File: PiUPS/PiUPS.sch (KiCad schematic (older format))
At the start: 101 parts, among them J1 USB_C_Receptacle_USB2.0, J2 Raspberry_Pi_2_3, J3 USB_A, J4 USB_B_Micro, J5 Screw_Terminal_01x02, J6 Screw_Terminal_01x02, Q1 IRF7404, Q2 IRF7404, Q3 IRLML2803TRPBF, Q4 IRF7404, Q5 IRF7404, Q6 IRLML2803TRPBF, Q7 IRLML2803TRPBF, SW1 MODE (JS102011SAQN), SW2 SW_MEC_5E, U1 LM393, U2 BQ25601, U3 TPS61088RHLR, U4 DS3231M

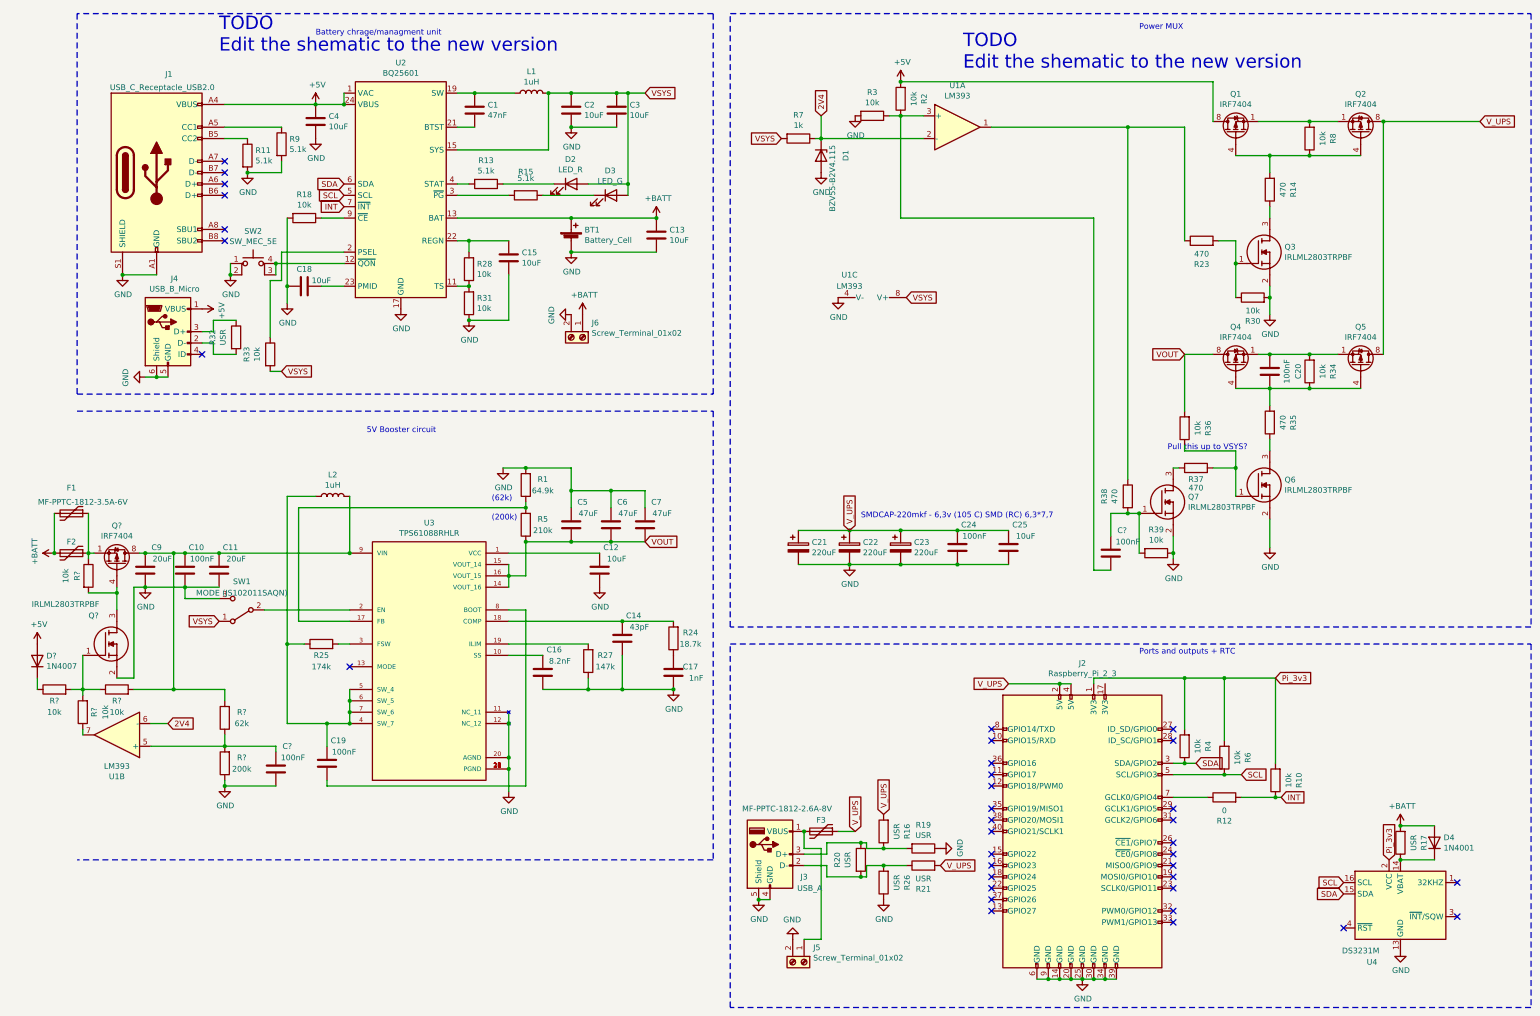
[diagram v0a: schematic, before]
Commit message: added almost final fixes for rev 0.1
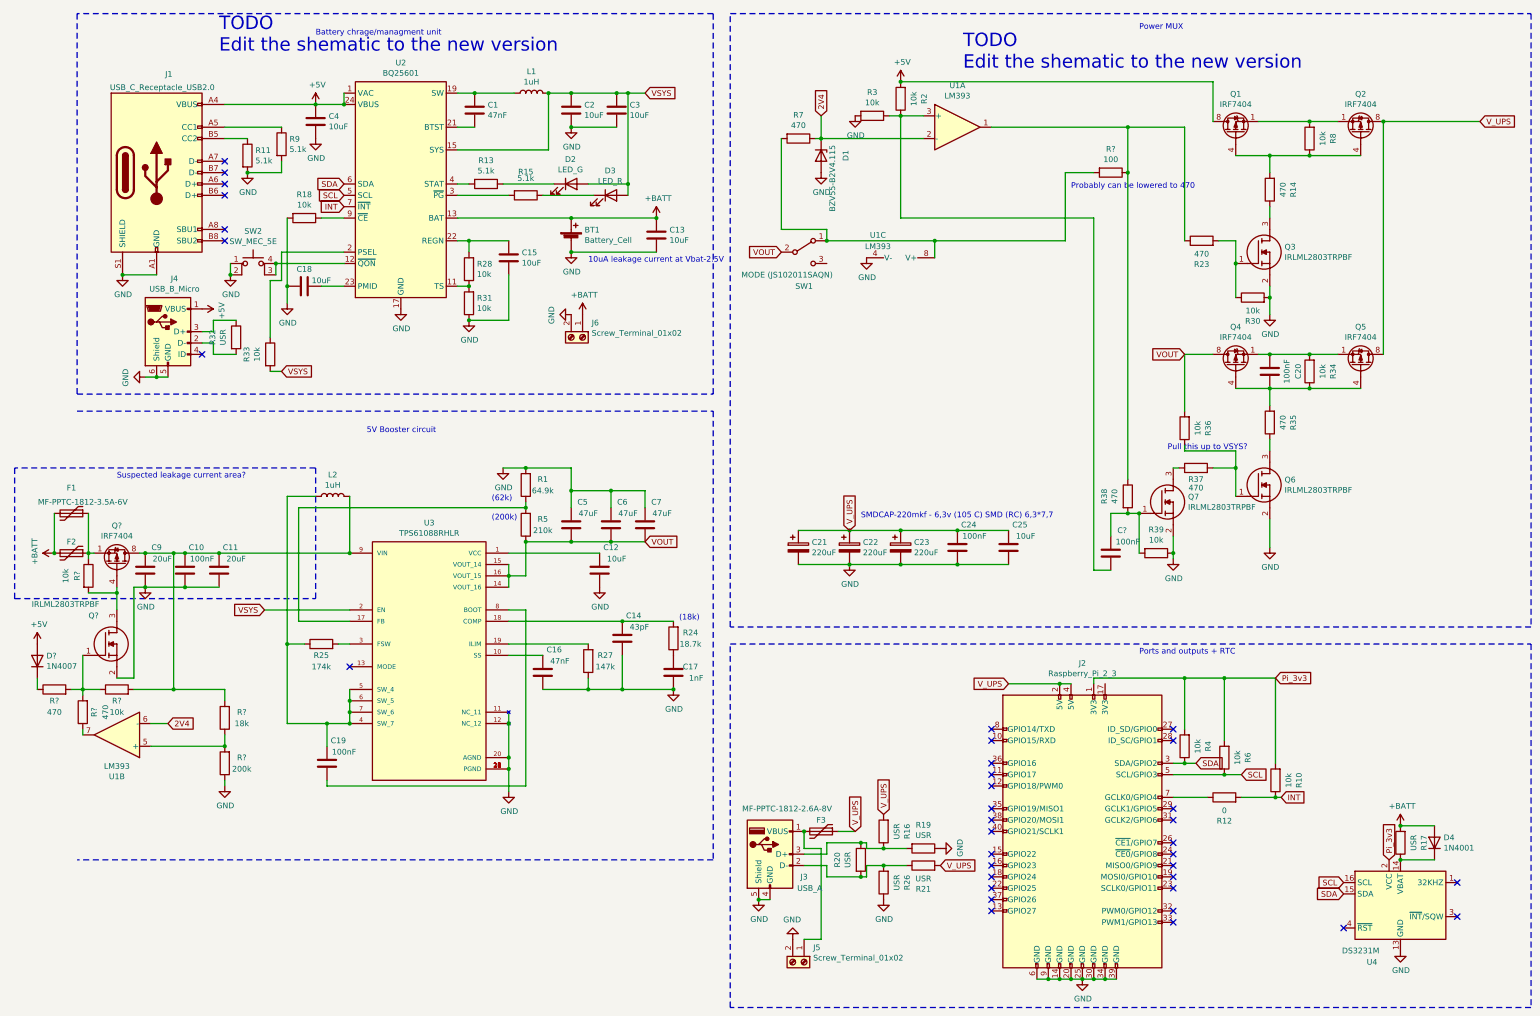
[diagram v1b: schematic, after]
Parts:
- removed C?: 100nF, Capacitor_SMD:C_0805_2012Metric_Pad1.18x1.45mm_HandSolder, symbol Device:C
- added R?: 100, Resistor_SMD:R_0805_2012Metric_Pad1.20x1.40mm_HandSolder, symbol Device:R
- C16: value 8.2nF -> 47nF
- D2: value LED_R -> LED_G
- D3: value LED_G -> LED_R
- R7: value 1k -> 470
- R?: value 62k -> 18k
- R? (x2): value 10k -> 470
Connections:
- net GND: no longer SW1.3 (C)
- net VOUT: now also SW1.2 (B)
- net VSYS: now also U3.2 (EN); no longer R7.2, SW1.1 (A), U1.8 (V+)
- net at R23.1, R38.1, U1.1: now also R?.1
- new net: R7.2, R?.2, SW1.1 (A), U1.8 (V+)
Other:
- note added: "(18k)\n"
- note added: "10uA leakage current at Vbat-2.5V"
- note added: "Probably can be lowered to 470"
- note added: "Suspected leakage current area?"
- moved on the sheet: SW1, U1C
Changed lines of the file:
@@
 P 5550 2500
 F 0 "D2" H 5543 2717 50  0000 C CNN
-F 1 "LED_R" H 5543 2626 50  0000 C CNN
+F 1 "LED_G" H 5543 2626 50  0000 C CNN
 F 2 "LED_SMD:LED_0805_2012Metric" H 5550 2500 50  0001 C CNN
 F 3 "~" H 5550 2500 50  0001 C CNN
@@
 P 5900 2600
 F 0 "D3" H 5893 2817 50  0000 C CNN
-F 1 "LED_G" H 5893 2726 50  0000 C CNN
+F 1 "LED_R" H 5893 2726 50  0000 C CNN
 F 2 "LED_SMD:LED_0805_2012Metric" H 5900 2600 50  0001 C CNN
 F 3 "~" H 5900 2600 50  0001 C CNN
@@
 P 5300 6800
 F 0 "C16" H 5400 7000 50  0000 C CNN
-F 1 "8.2nF" H 5450 6900 50  0000 C CNN
+F 1 "47nF" H 5450 6900 50  0000 C CNN
 F 2 "Capacitor_SMD:C_0805_2012Metric_Pad1.18x1.45mm_HandSolder" H 5338 6650 50  0001 C CNN
 F 3 "~" H 5300 6800 50  0001 C CNN
@@
 Wire Wire Line
 	6050 1700 6200 1700
-Text GLabel 2450 6350 0    50   Input ~ 0
-VSYS
 Wire Wire Line
 	2850 6250 3600 6250
-$Comp
-L Switch:SW_SPDT SW1
-U 1 1 612207C9
-P 2650 6250
-F 0 "SW1" H 2650 6000 50  0000 C CNN
-F 1 "MODE (JS102011SAQN)" H 2650 6100 50  0000 C CNN
-F 2 "Button_Switch_SMD:SW_SPDT_CK-JS102011SAQN" H 2650 6250 50  0001 C CNN
-F 3 "~" H 2650 6250 50  0001 C CNN
-	1    2650 6250
-	-1   0    0    1
-$EndComp
-Wire Wire Line
-	2450 6150 2150 6150
-Wire Wire Line
-	2150 6150 2150 6050
 Connection ~ 2150 6050
 Wire Notes Line
@@
 L Amplifier_Operational:LM358 U1
 U 3 1 612A3B8B
-P 8200 3600
-F 0 "U1" V 7900 3400 50  0000 C CNN
-F 1 "LM393" V 8000 3400 50  0000 C CNN
-F 2 "Package_SO:SOIC-8_3.9x4.9mm_P1.27mm" H 8200 3600 50  0001 C CNN
-F 3 "http://www.ti.com/lit/ds/symlink/lm2904-n.pdf" H 8200 3600 50  0001 C CNN
-	3    8200 3600
+P 8450 3250
+F 0 "U1" V 8150 3050 50  0000 C CNN
+F 1 "LM393" V 8250 3050 50  0000 C CNN
+F 2 "Package_SO:SOIC-8_3.9x4.9mm_P1.27mm" H 8450 3250 50  0001 C CNN
+F 3 "http://www.ti.com/lit/ds/symlink/lm2904-n.pdf" H 8450 3250 50  0001 C CNN
+	3    8450 3250
 	0    1    1    0
 $EndComp
@@
 	0    -1   -1   0
 $EndComp
-Text GLabel 7400 2100 0    50   Input ~ 0
-VSYS
 $Comp
 L power:GND #PWR09
@@
 P 7550 2100
 F 0 "R7" V 7343 2100 50  0000 C CNN
-F 1 "1k" V 7434 2100 50  0000 C CNN
+F 1 "470" V 7434 2100 50  0000 C CNN
 F 2 "Resistor_SMD:R_0805_2012Metric_Pad1.20x1.40mm_HandSolder" V 7480 2100 50  0001 C CNN
 F 3 "~" H 7550 2100 50  0001 C CNN
@@
 L power:GND #PWR010
 U 1 1 613779A5
-P 7900 3500
-F 0 "#PWR010" H 7900 3250 50  0001 C CNN
-F 1 "GND" H 7905 3327 50  0000 C CNN
-F 2 "" H 7900 3500 50  0001 C CNN
-F 3 "" H 7900 3500 50  0001 C CNN
-	1    7900 3500
-	1    0    0    -1
-$EndComp
-Text GLabel 8500 3500 2    50   Input ~ 0
-VSYS
+P 8150 3150
+F 0 "#PWR010" H 8150 2900 50  0001 C CNN
+F 1 "GND" H 8155 2977 50  0000 C CNN
+F 2 "" H 8150 3150 50  0001 C CNN
+F 3 "" H 8150 3150 50  0001 C CNN
+	1    8150 3150
+	1    0    0    -1
+$EndComp
 $Comp
 L Transistor_FET:IRF7404 Q2
@@
 Connection ~ 10550 5400
 Wire Wire Line
-	10450 5100 10450 2000
+	10450 5100 10450 2400
 Connection ~ 10450 2000
 Wire Wire Line
@@
 	-1   0    0    1
 $EndComp
-$Comp
-L Device:R R?
-U 1 1 6193474F
-P 2500 7200
-F 0 "R?" H 2350 7150 50  0000 C CNN
-F 1 "62k" H 2350 7250 50  0000 C CNN
-F 2 "Resistor_SMD:R_0805_2012Metric_Pad1.20x1.40mm_HandSolder" V 2430 7200 50  0001 C CNN
-F 3 "~" H 2500 7200 50  0001 C CNN
-	1    2500 7200
-	-1   0    0    1
-$EndComp
-Wire Wire Line
-	2500 7450 1850 7450
 Wire Wire Line
 	2500 7350 2500 7450
-Connection ~ 2500 7450
 $Comp
 L power:GND #PWR?
@@
 Wire Wire Line
 	2500 7800 2500 7750
-Wire Wire Line
-	2500 7050 2500 6950
-Wire Wire Line
-	2500 6950 2050 6950
 Connection ~ 2050 6950
 $Comp
@@
 P 1000 6950
 F 0 "R?" V 900 6950 50  0000 C CNN
-F 1 "10k" V 800 6950 50  0000 C CNN
+F 1 "470" V 800 6950 50  0000 C CNN
 F 2 "Resistor_SMD:R_0805_2012Metric_Pad1.20x1.40mm_HandSolder" V 930 6950 50  0001 C CNN
 F 3 "~" H 1000 6950 50  0001 C CNN
@@
 P 1250 7150
 F 0 "R?" V 1150 7150 50  0000 C CNN
-F 1 "10k" V 1050 7150 50  0000 C CNN
+F 1 "470" V 1050 7150 50  0000 C CNN
 F 2 "Resistor_SMD:R_0805_2012Metric_Pad1.20x1.40mm_HandSolder" V 1180 7150 50  0001 C CNN
 F 3 "~" H 1250 7150 50  0001 C CNN
@@
 	0    -1   -1   0
 $EndComp
-$Comp
-L Device:C C?
-U 1 1 617F0600
-P 2950 7650
-F 0 "C?" H 3050 7850 50  0000 C CNN
-F 1 "100nF" H 3100 7750 50  0000 C CNN
-F 2 "Capacitor_SMD:C_0805_2012Metric_Pad1.18x1.45mm_HandSolder" H 2988 7500 50  0001 C CNN
-F 3 "~" H 2950 7650 50  0001 C CNN
-	1    2950 7650
-	1    0    0    -1
-$EndComp
-Wire Wire Line
-	2500 7450 2950 7450
-Wire Wire Line
-	2950 7450 2950 7500
-Wire Wire Line
-	2950 7800 2500 7800
-Connection ~ 2500 7800
+Text GLabel 7400 3100 0    50   Input ~ 0
+VOUT
+$Comp
+L Device:R R?
+U 1 1 6189B0C4
+P 10300 2400
+F 0 "R?" V 10093 2400 50  0000 C CNN
+F 1 "100" V 10184 2400 50  0000 C CNN
+F 2 "Resistor_SMD:R_0805_2012Metric_Pad1.20x1.40mm_HandSolder" V 10230 2400 50  0001 C CNN
+F 3 "~" H 10300 2400 50  0001 C CNN
+	1    10300 2400
+	0    1    1    0
+$EndComp
+Connection ~ 10450 2400
+Wire Wire Line
+	10450 2400 10450 2000
+Text Notes 9950 2550 0    50   ~ 0
+Probably can be lowered to 470
+Text Notes 5700 3200 0    50   ~ 0
+10uA leakage current at Vbat-2.5V
+Wire Notes Line
+	650  5000 650  6150
+Wire Notes Line
+	650  6150 3300 6150
+Wire Notes Line
+	3300 6150 3300 5000
+Wire Notes Line
+	3300 5000 650  5000
+Text Notes 1550 5100 0    50   ~ 0
+Suspected leakage current area?
+Text Notes 6500 6350 0    50   ~ 0
+(18k)\n
+$Comp
+L Device:R R?
+U 1 1 6193474F
+P 2500 7200
+F 0 "R?" H 2350 7150 50  0000 C CNN
+F 1 "18k" H 2350 7250 50  0000 C CNN
+F 2 "Resistor_SMD:R_0805_2012Metric_Pad1.20x1.40mm_HandSolder" V 2430 7200 50  0001 C CNN
+F 3 "~" H 2500 7200 50  0001 C CNN
+	1    2500 7200
+	-1   0    0    1
+$EndComp
+Text GLabel 2850 6250 0    50   Input ~ 0
+VSYS
+$Comp
+L Switch:SW_SPDT SW1
+U 1 1 612207C9
+P 7600 3100
+F 0 "SW1" H 7600 2800 50  0000 C CNN
+F 1 "MODE (JS102011SAQN)" H 7450 2900 50  0000 C CNN
+F 2 "Button_Switch_SMD:SW_SPDT_CK-JS102011SAQN" H 7600 3100 50  0001 C CNN
+F 3 "~" H 7600 3100 50  0001 C CNN
+	1    7600 3100
+	1    0    0    -1
+$EndComp
+Wire Wire Line
+	2050 6950 2500 6950
+Wire Wire Line
+	2500 6950 2500 7050
+Wire Wire Line
+	1850 7450 2500 7450
+Connection ~ 2500 7450
+Wire Wire Line
+	7800 3000 8750 3000
+Wire Wire Line
+	8750 3000 8750 3150
+Wire Wire Line
+	7400 2100 7400 2900
+Wire Wire Line
+	7400 2900 7800 2900
+Wire Wire Line
+	7800 2900 7800 3000
+Connection ~ 7800 3000
+Wire Wire Line
+	10150 2400 9900 2400
+Wire Wire Line
+	9900 2400 9900 3000
+Wire Wire Line
+	9900 3000 8750 3000
+Connection ~ 8750 3000
 $EndSCHEMATC

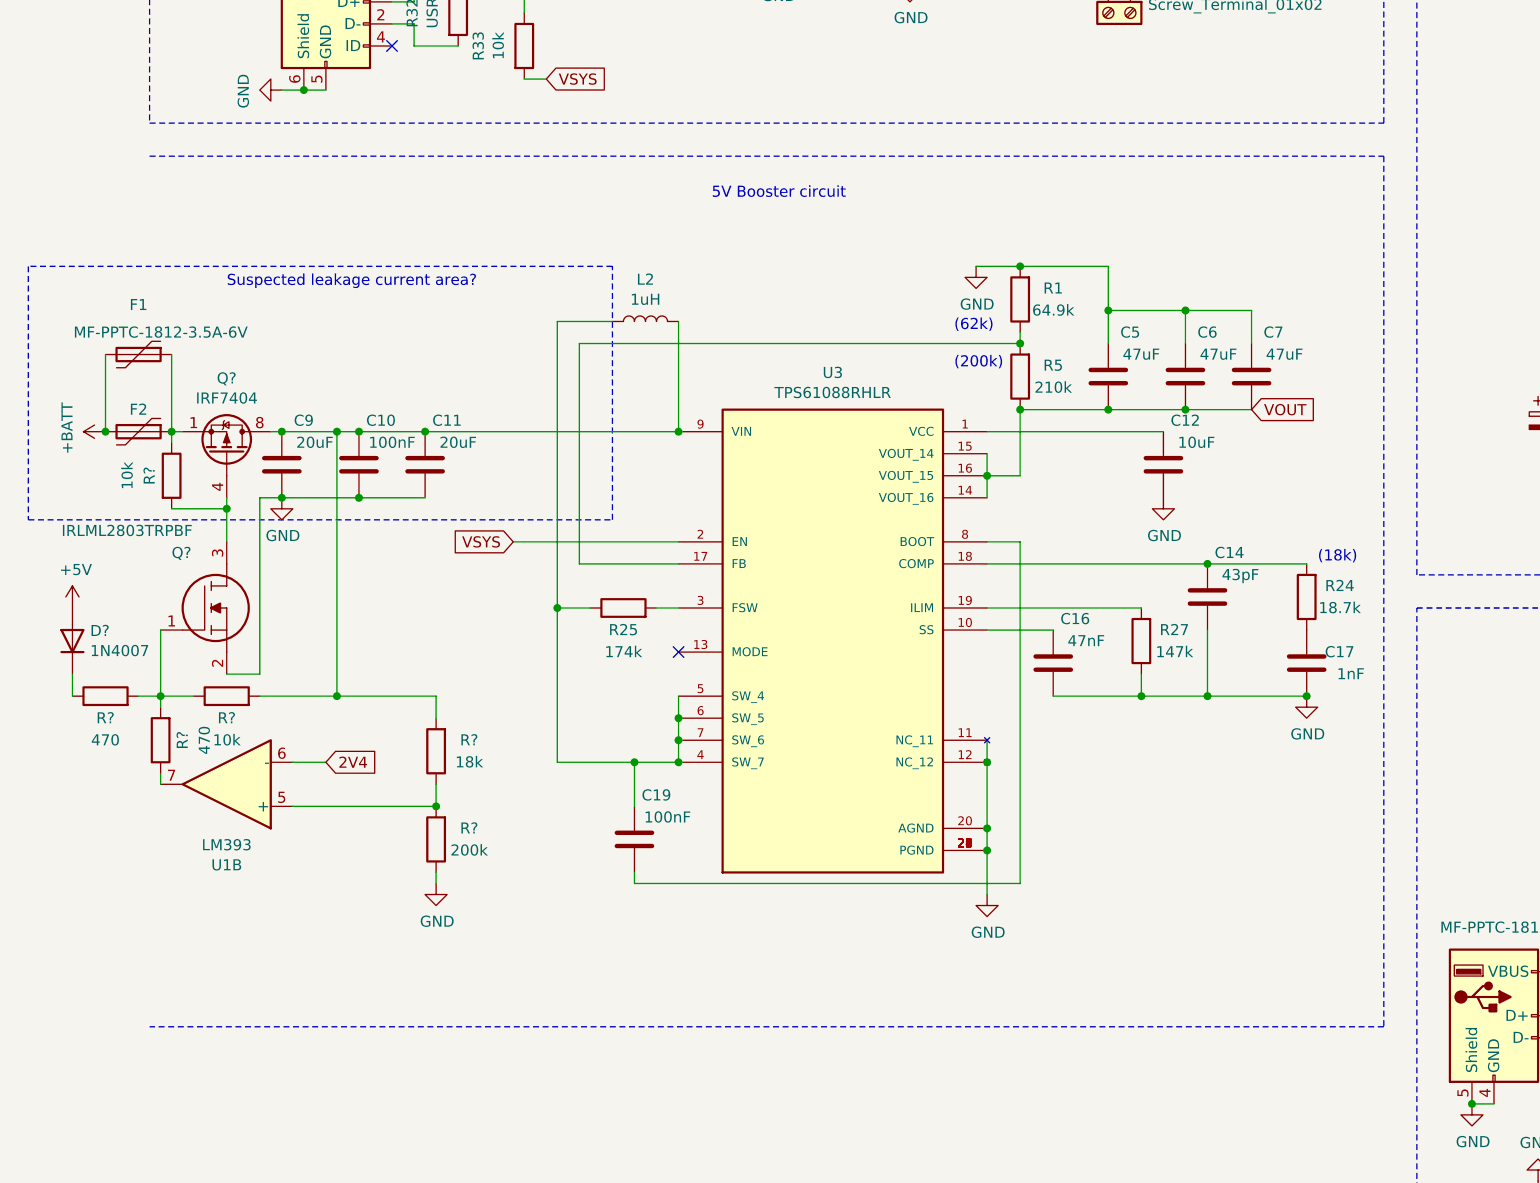
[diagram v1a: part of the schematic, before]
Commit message: tidied up schematic
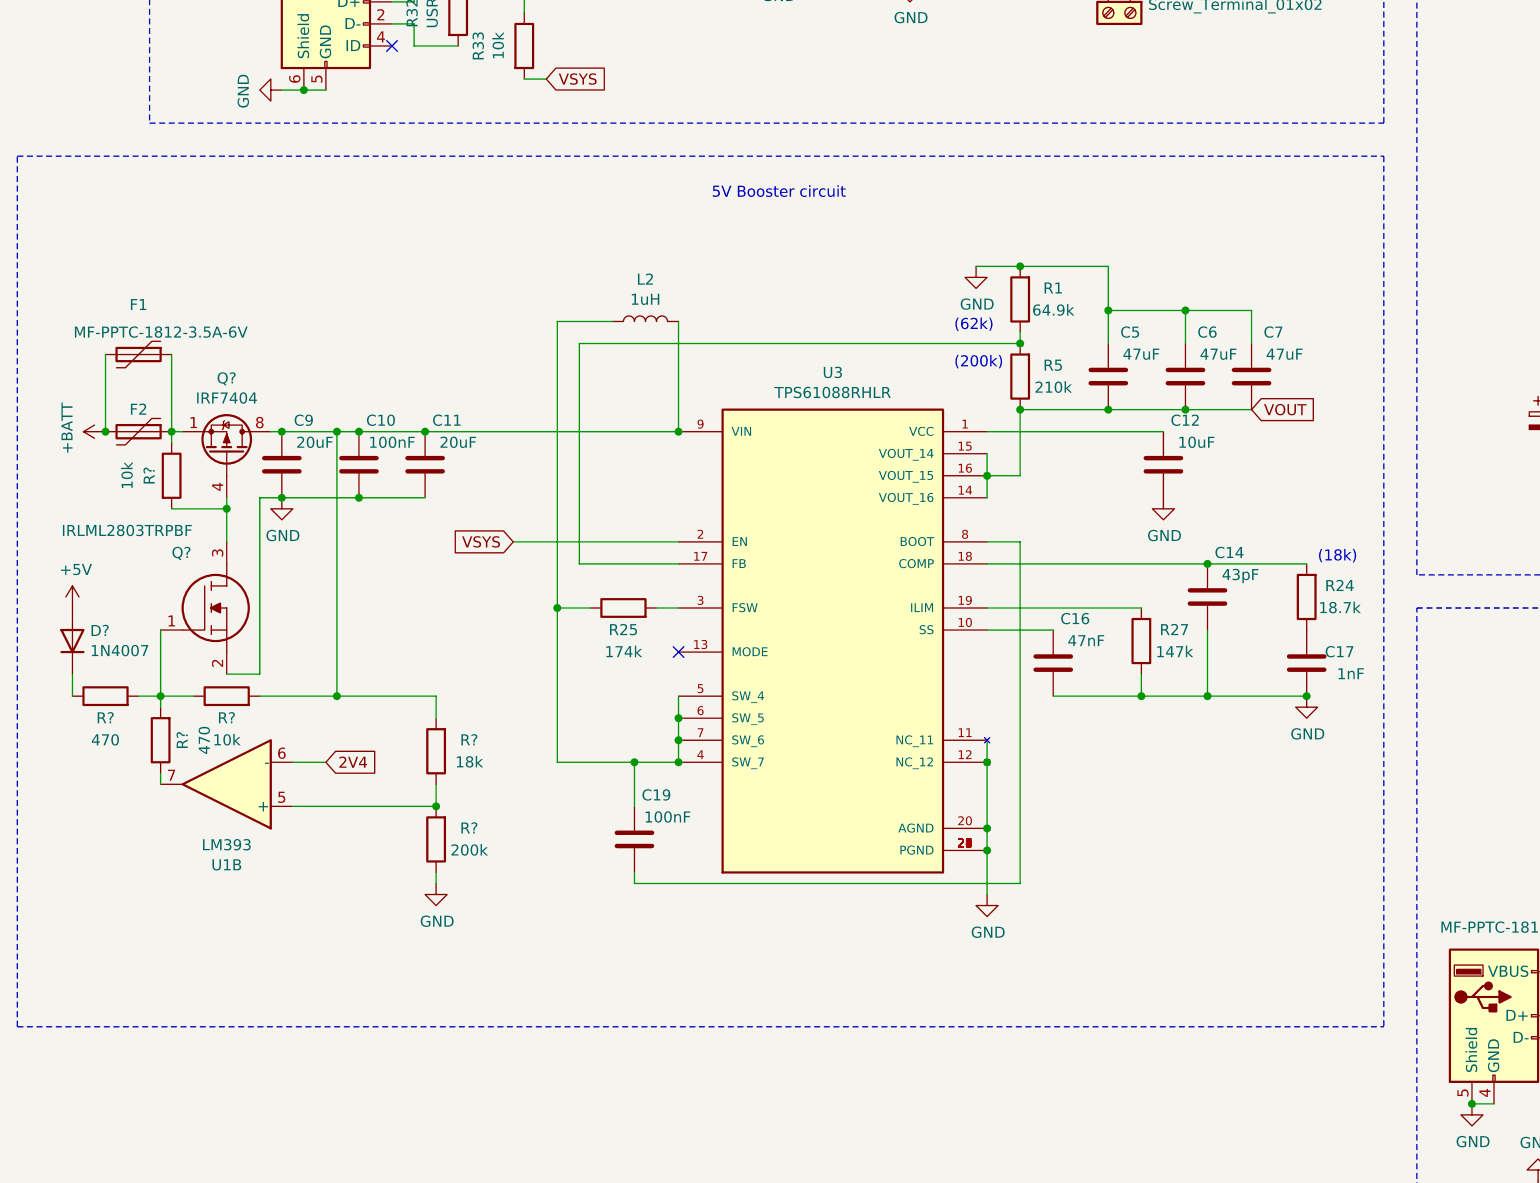
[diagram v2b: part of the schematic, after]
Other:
- note removed: "Suspected leakage current area?"
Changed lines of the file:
@@
 Connection ~ 2150 6050
 Wire Notes Line
-	1200 4500 6800 4500
-Wire Notes Line
 	6800 4500 6800 8450
-Wire Notes Line
-	6800 8450 1200 8450
 Text Notes 3750 4700 0    50   ~ 0
 5V Booster circuit
@@
 Text Notes 5700 3200 0    50   ~ 0
 10uA leakage current at Vbat-2.5V
-Wire Notes Line
-	650  5000 650  6150
-Wire Notes Line
-	650  6150 3300 6150
-Wire Notes Line
-	3300 6150 3300 5000
-Wire Notes Line
-	3300 5000 650  5000
-Text Notes 1550 5100 0    50   ~ 0
-Suspected leakage current area?
 Text Notes 6500 6350 0    50   ~ 0
 (18k)\n
@@
 	9900 3000 8750 3000
 Connection ~ 8750 3000
+Wire Notes Line
+	600  8450 600  4500
+Wire Notes Line
+	600  4500 6800 4500
+Wire Notes Line
+	600  8450 6800 8450
 $EndSCHEMATC
